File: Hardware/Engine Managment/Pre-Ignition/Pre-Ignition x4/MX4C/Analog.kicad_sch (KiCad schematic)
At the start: 57 parts, among them J4 Map/Baro Sensor Socket, J6 VR_Header, Q10 AO3400A, Q11 AO3400A, Q9 AO3400A, U1 SRV05-4-P-T7, U4 SRV05-4-P-T7, U5 SRV05-4-P-T7

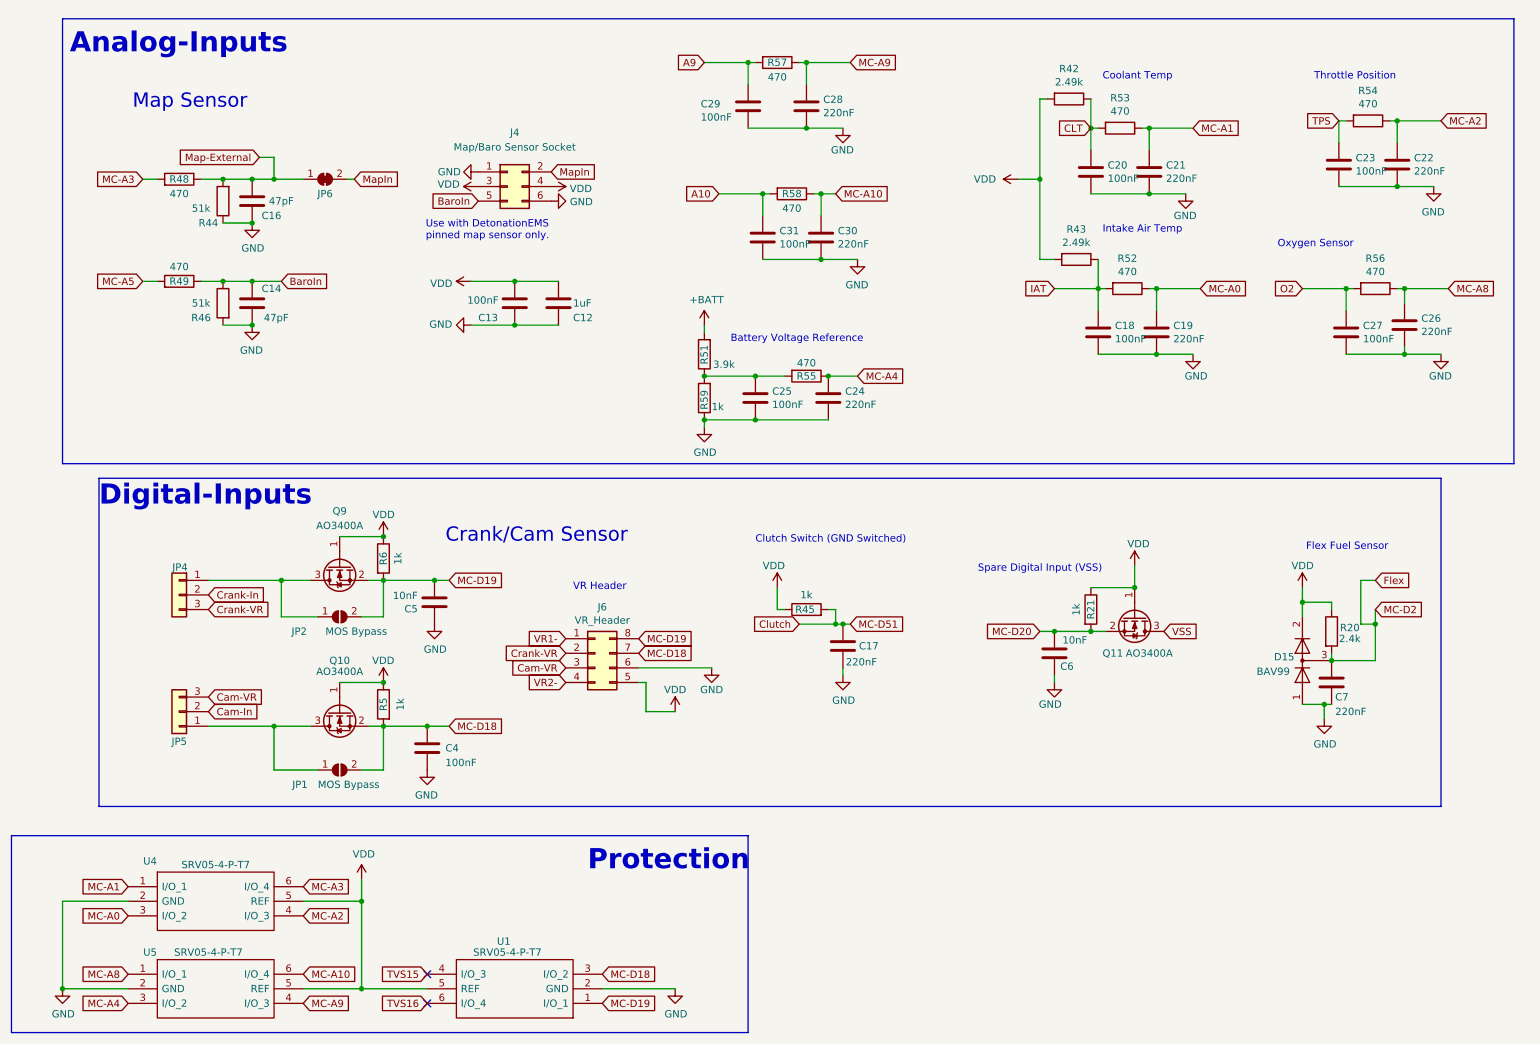
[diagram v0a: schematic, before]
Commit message: Structure Update
MX2 - RevB Upload
MX4B-2 - KiCad Version update (no changes)
MX4C - Organized Schematic, Minor layout change
Engine Simulator 8 Channel - Organized Schematic (no changes)
PMAP-M - Map Sensor Breakout for MX4C
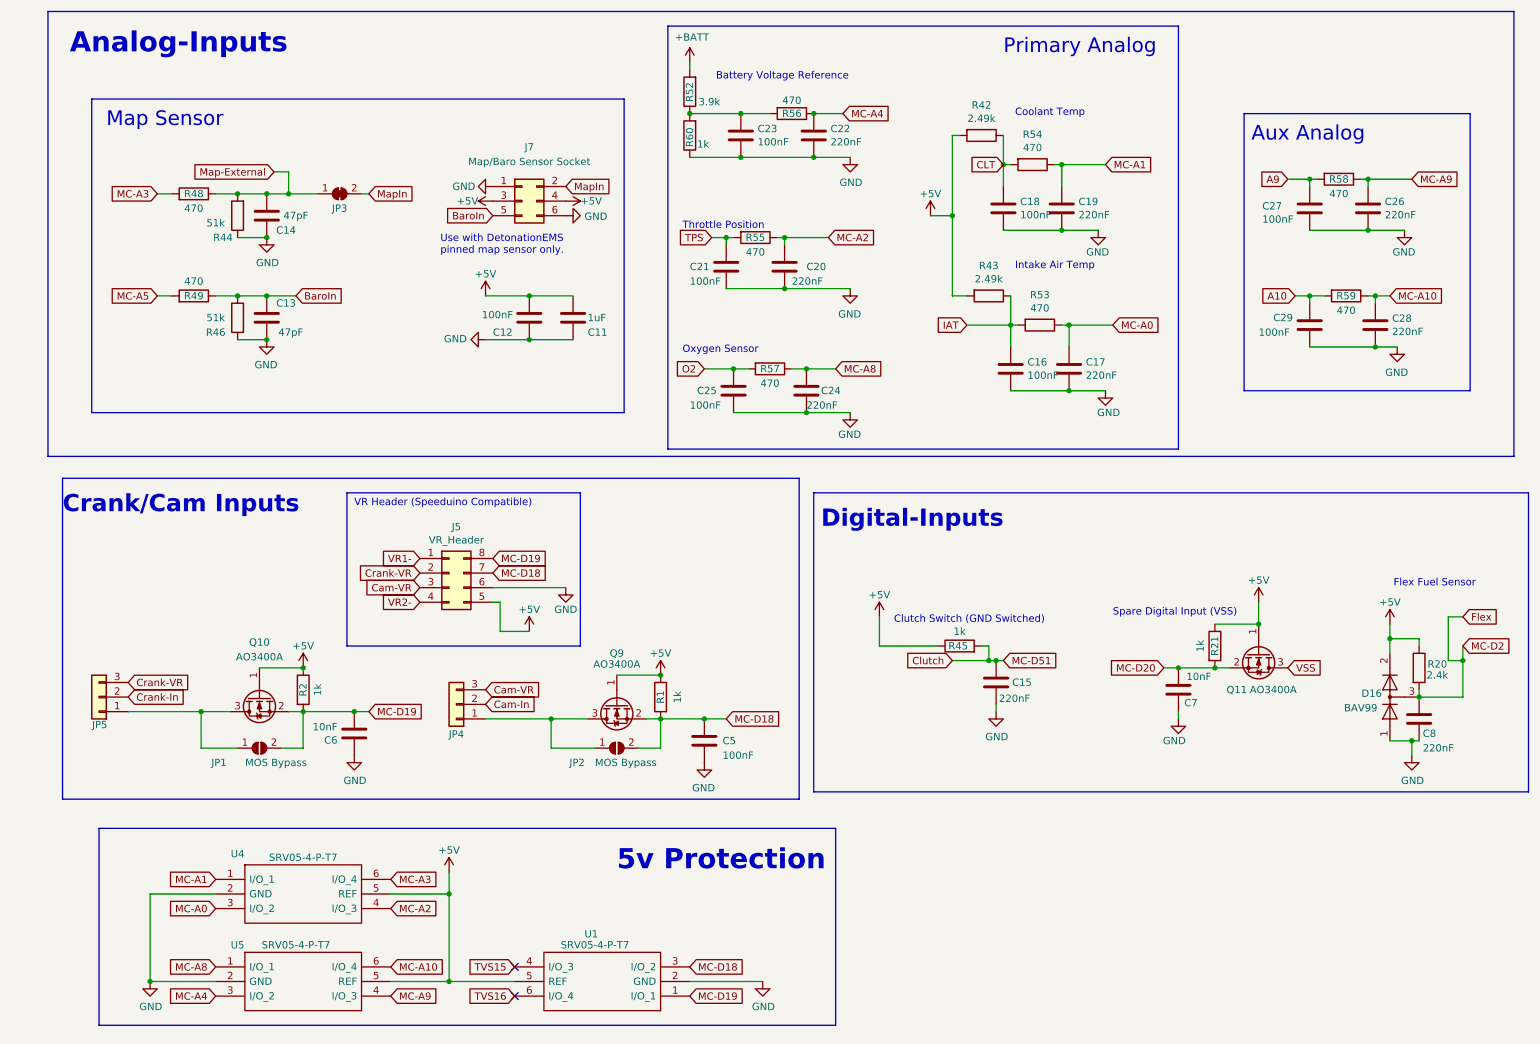
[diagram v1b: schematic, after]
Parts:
- renumbered C12 to C11, C13 to C12, C14 to C13, C16 to C14, C17 to C15, C18 to C16, C19 to C17, C20 to C18, C21 to C19, C22 to C20, C23 to C21, C24 to C22, C25 to C23, C26 to C24, C27 to C25, C28 to C26, C29 to C27, C30 to C28, C31 to C29, C4 to C5, C5 to C6, C6 to C7, C7 to C8, D15 to D16, J6 to J5, J4 to J7, JP2 to JP1, JP1 to JP2, JP6 to JP3, JP5 to JP4, JP4 to JP5, Q9 to Q10, Q10 to Q9, R5 to R1, R6 to R2, R51 to R52, R52 to R53, R53 to R54, R54 to R55, R55 to R56, R56 to R57, R57 to R58, R58 to R59, R59 to R60
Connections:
- net VDD renamed +5V
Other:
- note added: "5v Protection"
- note added: "Aux Analog"
- note added: "Crank/Cam Inputs"
- note added: "Primary Analog"
- note added: "VR Header (Speeduino Compatible)"
- note removed: "Crank/Cam Sensor"
- note removed: "Protection"
- note removed: "VR Header"
- moved on the sheet: C11, C12, C13, C14, C15, C16, C17, C18, C19, C20, C21, C22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
